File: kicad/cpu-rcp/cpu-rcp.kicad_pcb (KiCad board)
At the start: 2 copper layers, 86.4 x 63.5 mm, 79 parts, among them P1 RDRAM-EDGE, P5 NINTENDO-64_PINHEAD-25X2, SW1 Reset, U1 9480F, U10 CPU-NUS, U6 PIF-NUS, U7 MX8330, U9 RCP-NUS, X1 14.318MHz

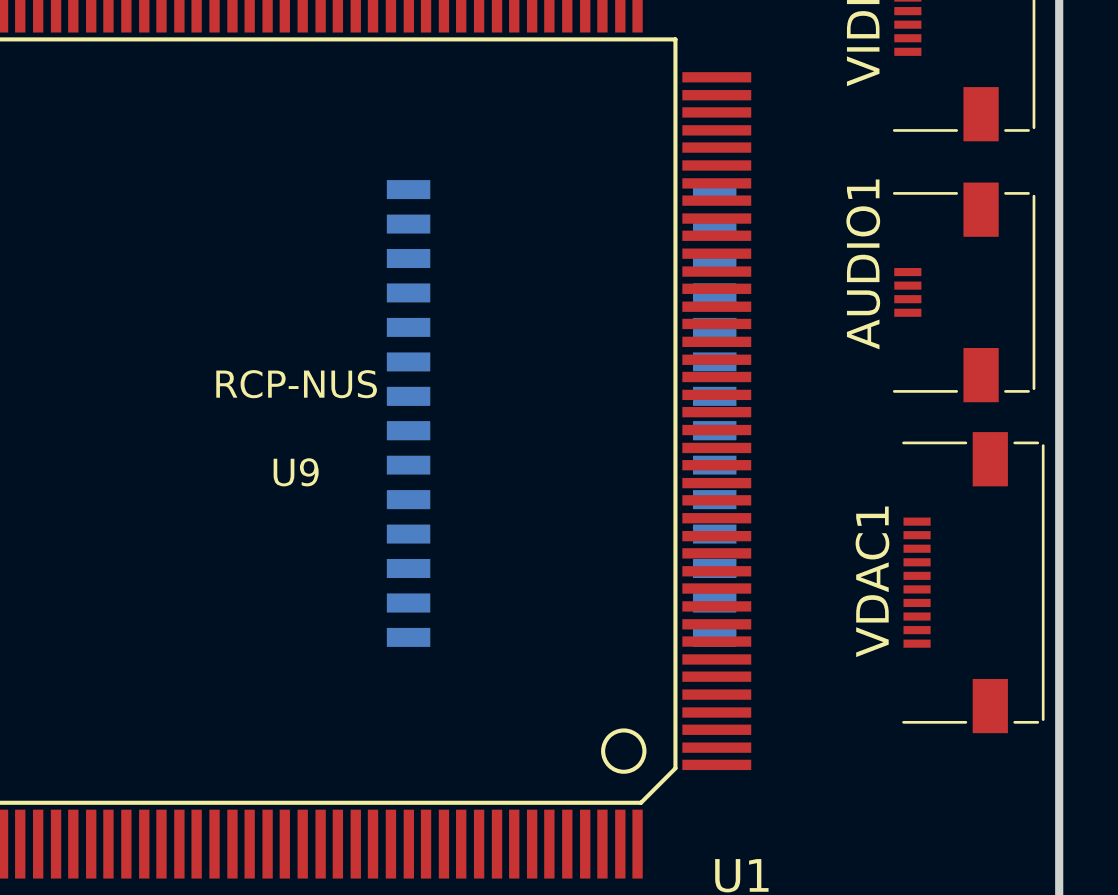
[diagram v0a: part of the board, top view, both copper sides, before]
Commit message: Work in progress, updated 3D shapes
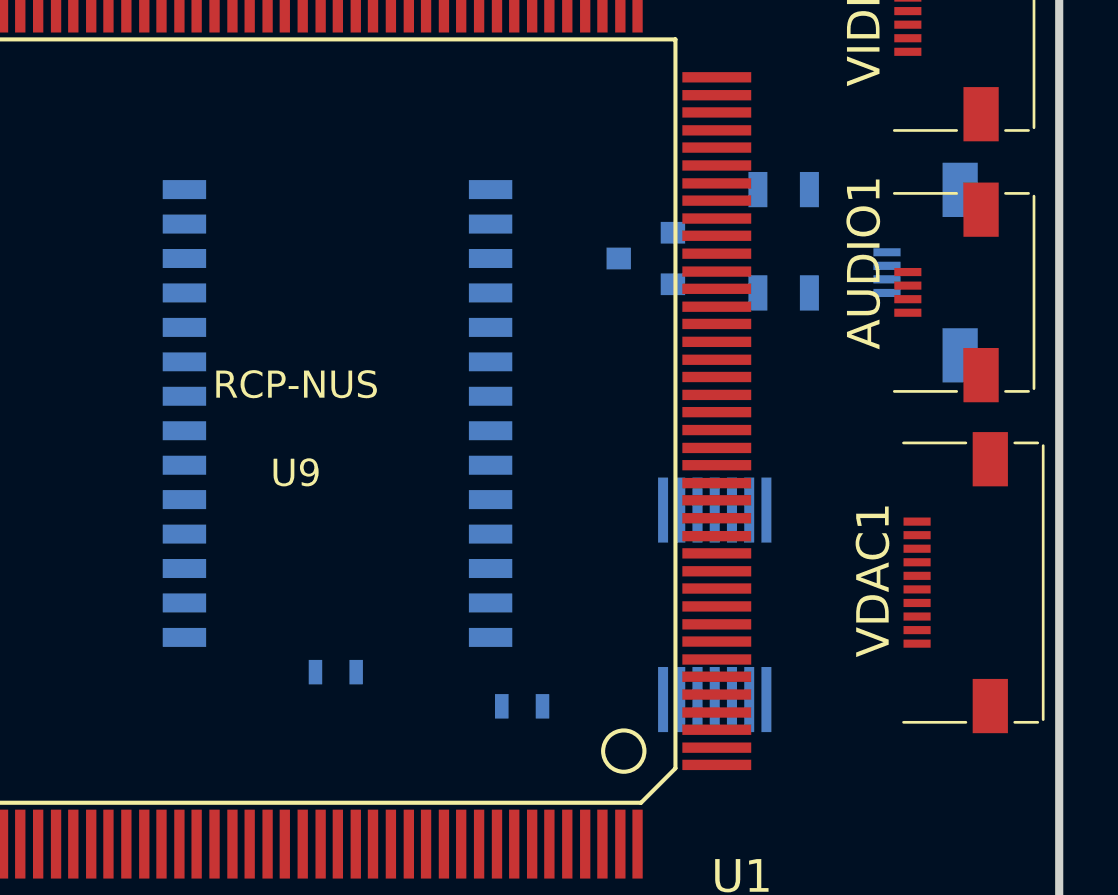
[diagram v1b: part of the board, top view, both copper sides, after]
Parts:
- added DA1: BAC54, n64:D_SOT-23_AAK, B.Cu at (96.5, 45.7)
- added FIL2: 3.3uH, n64:L_0805, B.Cu at (101.6, 47.0)
- added FIL4: 3.3uH, n64:L_0805, B.Cu at (101.6, 43.2)
- added JOY1: JOY OUT, n64:connector-molex-505110-0492, B.Cu at (105.9, 45.5)
- added R37: 750R, n64:R_0603, B.Cu at (92.0, 62.2)
- added R38: 750R, n64:R_0603, B.Cu at (85.1, 61.0)
- added U8: LC125, n64:ssop-14, B.Cu at (99.1, 58.4)
- moved U6 8.26 mm to (85.1, 52.1)
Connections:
- C144 pad 1: Net-(C144-Pad1) -> GND
- C144 pad 2: GND -> Net-(C144-Pad2)
- DCIN1 pad 4: ENABLE -> +3V3
- R36 pad 1: Net-(C144-Pad1) -> ENABLE
- R36 pad 2: ENABLE -> Net-(C144-Pad2)
- U6 pad 15: Net-(U6-Pad15) -> JOY1_DATA
- U6 pad 17: Net-(U6-Pad17) -> JOY2_DATA
- U7 pad 7: Net-(C144-Pad1) -> Net-(C144-Pad2)
